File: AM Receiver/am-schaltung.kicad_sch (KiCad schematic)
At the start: 43 parts, among them IC100 SA612AD, IC103 TDA1072AT, P100 10k 25% Trimmer, Q100 MMBFJ310LT3G, Q101 MMBFJ310LT3G

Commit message: Updated User.drawing information and Design Review
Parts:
- FL100: ProcurementNote (none) -> Legacy/EOL risk for SFZ455A/SFZLA455KN2A-B0; verify stock/l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
- IC100: ProcurementNote (none) -> Legacy/EOL risk for SA612AD/01,118; verify stock/lifecycle 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
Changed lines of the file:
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@@
+			)
+		)
+		(property "ProcurementNote" "Legacy/EOL risk for SA612AD/01,118; verify stock/lifecycle and approved substitute before build."
+			(at 120.65 102.87 0)
+			(hide yes)
+			(show_name no)
+			(do_not_autoplace no)
+			(effects
+				(font
+					(size 1.27 1.27)
+				)
 			)
 		)
@@
 			(at 193.04 101.6 0)
 			(hide yes)
+			(show_name no)
+			(do_not_autoplace no)
+			(effects
+				(font
+					(size 1.27 1.27)
+				)
+			)
+		)
+		(property "ProcurementNote" "Legacy/EOL risk for SFZ455A/SFZLA455KN2A-B0; verify stock/lifecycle or compatible 455 kHz ceramic IF filter before build."
+			(at 193.04 101.6 0)
+			(hide yes)

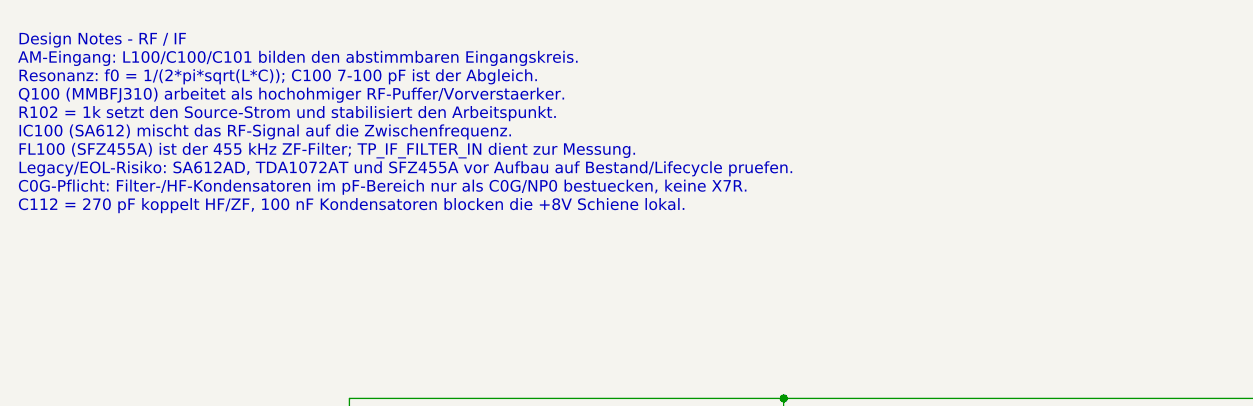
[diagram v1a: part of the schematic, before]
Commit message: Updated Design notes in schematic
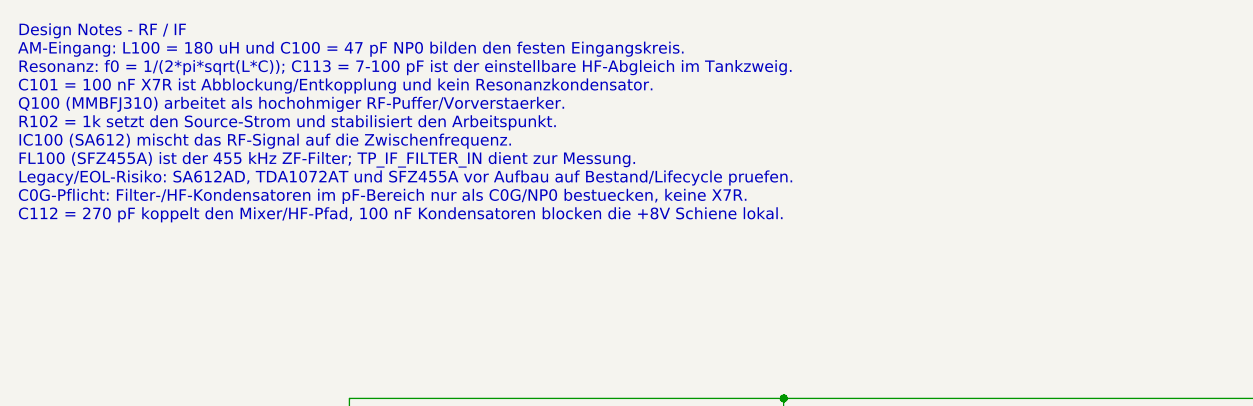
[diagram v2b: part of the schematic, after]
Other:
- note added: "Design Notes - RF / IF AM-Eingang: L100 = 180 uH und C100 = 47 pF NP0 bilden den festen Eingangskreis. Resonanz: f0 = 1/(2*pi*sqrt(L*C)); C113 = 7-100 pF ist der einstellbare HF-Abgleich im Tankzweig. C101 = 100 nF X7R ist Abblockung/Entkopplung und kein Resonanzkondensator. Q100 (MMBFJ310) arbeitet als hochohmiger RF-Puffer/Vorverstaerker. R102 = 1k setzt den Source-Strom und stabilisiert den Ar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"
- note removed: "Design Notes - RF / IF AM-Eingang: L100/C100/C101 bilden den abstimmbaren Eingangskreis. Resonanz: f0 = 1/(2*pi*sqrt(L*C)); C100 7-100 pF ist der Abgleich. Q100 (MMBFJ310) arbeitet als hochohmiger RF-Puffer/Vorverstaerker. R102 = 1k setzt den Source-Strom und stabilisiert den Arbeitspunkt. IC100 (SA612) mischt das RF-Signal auf die Zwischenfrequenz. FL100 (SFZ455A) ist der 455 kHz ZF-Filter; TP_I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"
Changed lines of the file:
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@@
 		(comment 3 "T. Brown")
 	)
-	(text "Design Notes - RF / IF\nAM-Eingang: L100/C100/C101 bilden den abstimmbaren Eingangskreis.\nResonanz: f0 = 1/(2*pi*sqrt(L*C)); C100 7-100 pF ist der Abgleich.\nQ100 (MMBFJ310) arbeitet als hochohmiger RF-Puffer/Vorverstaerker.\nR102 = 1k setzt den Source-Strom und stabilisiert den Arbeitspunkt.\nIC100 (SA612) mischt das RF-Signal auf die Zwischenfrequenz.\nFL100 (SFZ455A) ist der 455 kHz ZF-Filter; TP_IF_FILTER_IN dient zur Messung.\nLegacy/EOL-Risiko: SA612AD, TDA1072AT und SFZ455A vor Aufbau auf Bestand/Lifecycle pruefen.\nC0G-Pflicht: Filter-/HF-Kondensatoren im pF-Bereich nur als C0G/NP0 bestuecken, keine X7R.\nC112 = 270 pF koppelt HF/ZF, 100 nF Kondensatoren blocken die +8V Schiene lokal."
+	(text "Design Notes - RF / IF\nAM-Eingang: L100 = 180 uH und C100 = 47 pF NP0 bilden den festen Eingangskreis.\nResonanz: f0 = 1/(2*pi*sqrt(L*C)); C113 = 7-100 pF ist der einstellbare HF-Abgleich im Tankzweig.\nC101 = 100 nF X7R ist Abblockung/Entkopplung und kein Resonanzkondensator.\nQ100 (MMBFJ310) arbeitet als hochohmiger RF-Puffer/Vorverstaerker.\nR102 = 1k setzt den Source-Strom und stabilisiert den Arbeitspunkt.\nIC100 (SA612) mischt das RF-Signal auf die Zwischenfrequenz.\nFL100 (SFZ455A) ist der 455 kHz ZF-Filter; TP_IF_FILTER_IN dient zur Messung.\nLegacy/EOL-Risiko: SA612AD, TDA1072AT und SFZ455A vor Aufbau auf Bestand/Lifecycle pruefen.\nC0G-Pflicht: Filter-/HF-Kondensatoren im pF-Bereich nur als C0G/NP0 bestuecken, keine X7R.\nC112 = 270 pF koppelt den Mixer/HF-Pfad, 100 nF Kondensatoren blocken die +8V Schiene lokal."
 		(exclude_from_sim no)
 		(at 35.56 34.29 0)
